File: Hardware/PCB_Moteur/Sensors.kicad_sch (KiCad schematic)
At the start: 18 parts, among them J18 Screw_Terminal_01x04, J3 Screw_Terminal_01x04, U8 INA125UA/2K5, U9 MAX6612MXK

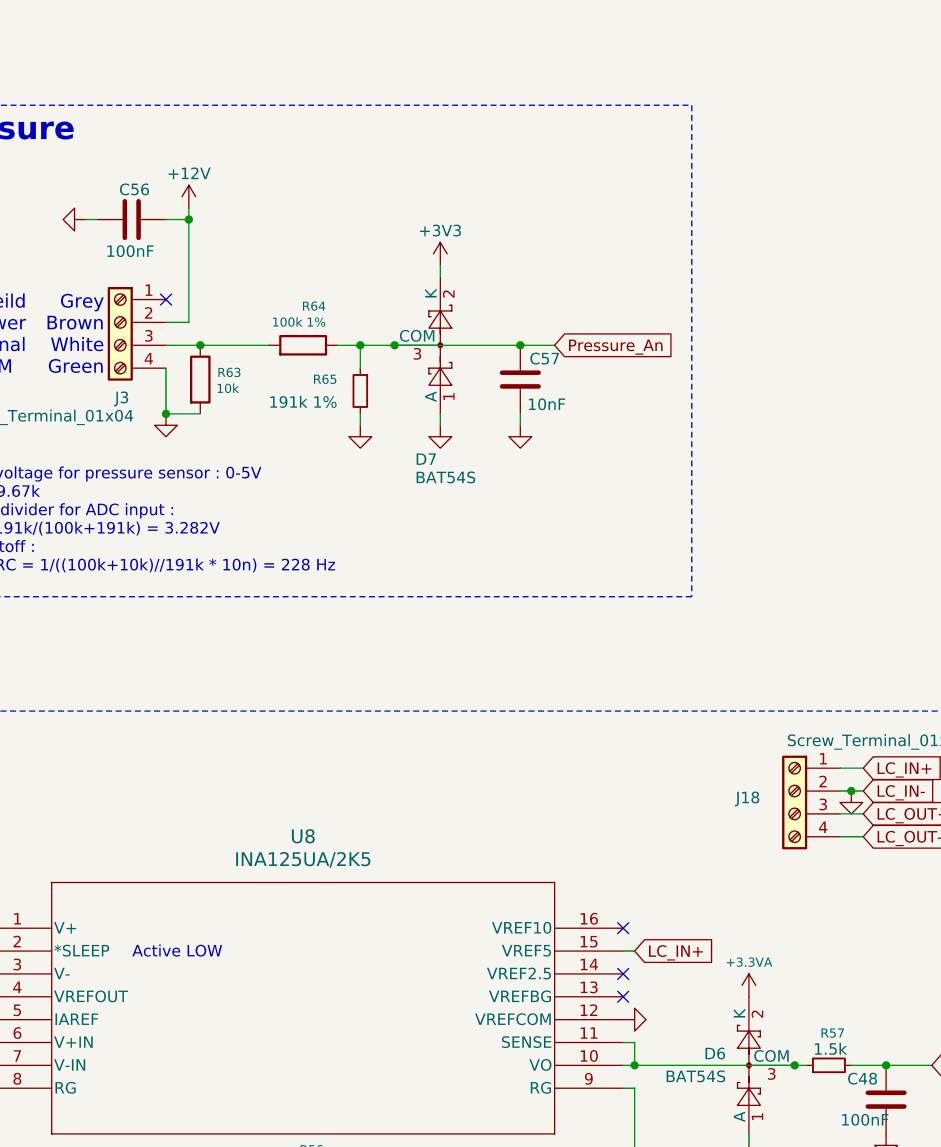
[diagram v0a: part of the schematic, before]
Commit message: wip: new pressure et fix alim
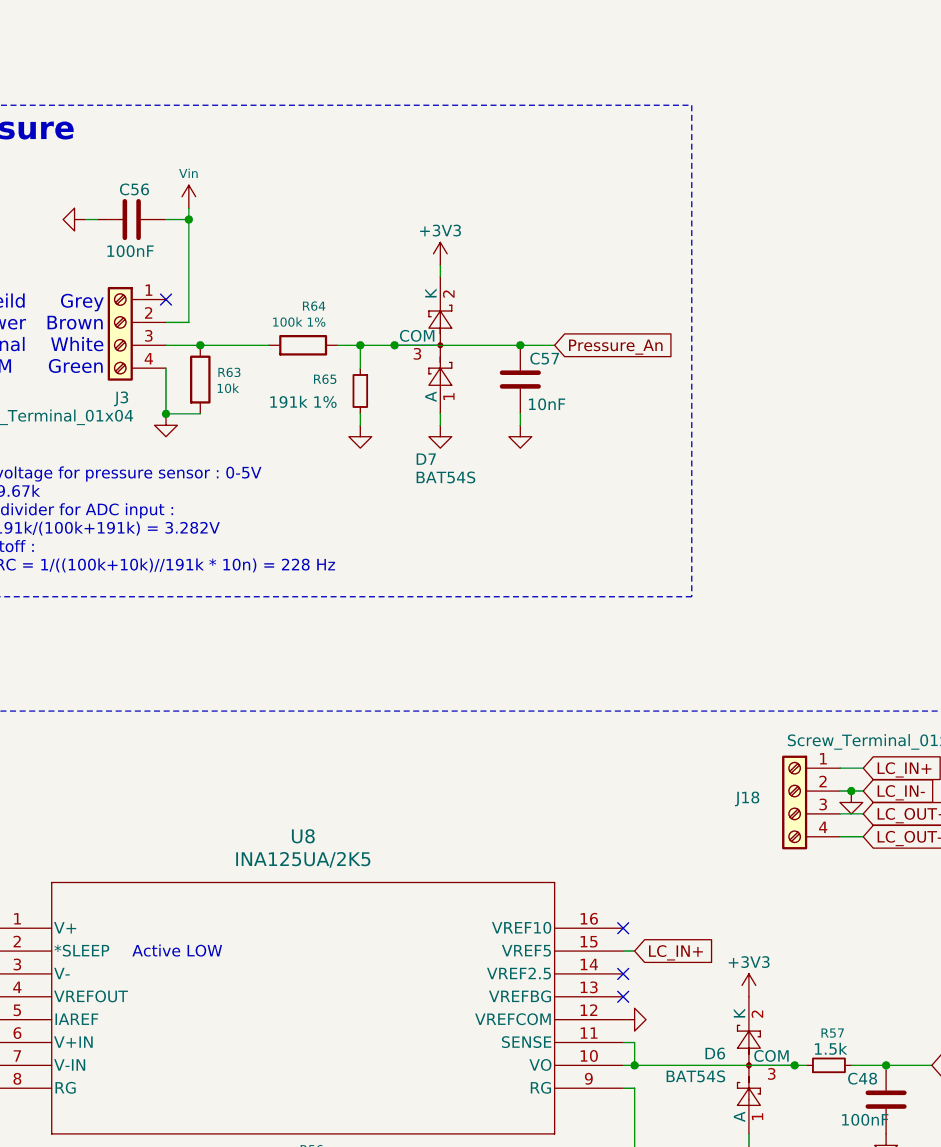
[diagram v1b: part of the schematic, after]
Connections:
- net +12V is gone; now on net Vin: C56.2, J3.2 (Pin_2)
- net +3.3VA is gone; now on net +3V3: D6.2 (K)
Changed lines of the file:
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@@
 	)
 	(symbol
-		(lib_id "power:+3.3VA")
+		(lib_id "power:+3V3")
 		(at 127 133.35 0)
-		(unit 1)
-		(exclude_from_sim no)
-		(in_bom yes)
-		(on_board yes)
-		(dnp no)
-		(property "Reference" "#PWR075"
+		(mirror y)
+		(unit 1)
+		(exclude_from_sim no)
+		(in_bom yes)
+		(on_board yes)
+		(dnp no)
+		(property "Reference" "#PWR037"
 			(at 127 137.16 0)
 			(effects
 				(font
-					(size 1 1)
-				)
-				(hide yes)
-			)
-		)
-		(property "Value" "+3.3VA"
+					(size 1.27 1.27)
+				)
+				(hide yes)
+			)
+		)
+		(property "Value" "+3V3"
 			(at 127 129.54 0)
 			(effects
 				(font
-					(size 1 1)
+					(size 1.27 1.27)
 				)
 			)
@@
 			(effects
 				(font
-					(size 1 1)
+					(size 1.27 1.27)
 				)
 				(hide yes)
@@
 			(effects
 				(font
-					(size 1 1)
-				)
-				(hide yes)
-			)
-		)
-		(property "Description" ""
+					(size 1.27 1.27)
+				)
+				(hide yes)
+			)
+		)
+		(property "Description" "Power symbol creates a global label with name \"+3V3\""
 			(at 127 133.35 0)
 			(effects
@@
 					(size 1.27 1.27)
 				)
-			)
-		)
-		(pin "1"
-		)
-		(instances
-			(project "PCB_moteur"
-				(path "/b0d87684-7b1c-41d8-8358-755aa327573e/f31687d3-ca84-4d71-914a-32b6c2b363a9"
-					(reference "#PWR075")
+				(hide yes)
+			)
+		)
+		(pin "1"
+		)
+		(instances
+			(project "PCB_moteur"
+				(path "/b0d87684-7b1c-41d8-8358-755aa327573e/f31687d3-ca84-4d71-914a-32b6c2b363a9"
+					(reference "#PWR037")
 					(unit 1)
 				)
@@
 	)
 	(symbol
-		(lib_name "+12V_1")
-		(lib_id "power:+12V")
-		(at 64.77 45.72 0)
-		(unit 1)
-		(exclude_from_sim no)
-		(in_bom yes)
-		(on_board yes)
-		(dnp no)
-		(property "Reference" "#PWR0146"
-			(at 64.77 49.53 0)
-			(effects
-				(font
-					(size 1.27 1.27)
-				)
-				(hide yes)
-			)
-		)
-		(property "Value" "+12V"
-			(at 64.77 41.91 0)
-			(effects
-				(font
-					(size 1.27 1.27)
-				)
-			)
-		)
-		(property "Footprint" ""
-			(at 64.77 45.72 0)
-			(effects
-				(font
-					(size 1.27 1.27)
-				)
-				(hide yes)
-			)
-		)
-		(property "Datasheet" ""
-			(at 64.77 45.72 0)
-			(effects
-				(font
-					(size 1.27 1.27)
-				)
-				(hide yes)
-			)
-		)
-		(property "Description" "Power symbol creates a global label with name \"+12V\""
-			(at 64.77 45.72 0)
-			(effects
-				(font
-					(size 1.27 1.27)
-				)
-				(hide yes)
-			)
-		)
-		(pin "1"
-		)
-		(instances
-			(project "PCB_moteur"
-				(path "/b0d87684-7b1c-41d8-8358-755aa327573e/f31687d3-ca84-4d71-914a-32b6c2b363a9"
-					(reference "#PWR0146")
-					(unit 1)
-				)
-			)
-		)
-	)
-	(symbol
 		(lib_id "power:GND")
 		(at 101.6 69.85 0)
@@
 					(unit 1)
 				)
+			)
+		)
+	)
+	(symbol
+		(lib_id "power:+12V")
+		(at 64.77 45.72 0)
+		(unit 1)
+		(exclude_from_sim no)
+		(in_bom yes)
+		(on_board yes)
+		(dnp no)
+		(property "Reference" "#PWR07"
+			(at 64.77 49.53 0)
+			(effects
+				(font
+					(size 1 1)
+				)
+				(hide yes)
+			)
+		)
+		(property "Value" "Vin"
+			(at 64.77 41.91 0)
+			(effects
+				(font
+					(size 1 1)
+				)
+			)
+		)
+		(property "Footprint" ""
+			(at 64.77 45.72 0)
+			(effects
+				(font
+					(size 1 1)
+				)
+				(hide yes)
+			)
+		)
+		(property "Datasheet" ""
+			(at 64.77 45.72 0)
+			(effects
+				(font
+					(size 1 1)
+				)
+				(hide yes)
+			)
+		)
+		(property "Description" ""
+			(at 64.77 45.72 0)
+			(effects
+				(font
+					(size 1.27 1.27)
+				)
+				(hide yes)
+			)
+		)
+		(pin "1"
+		)
+		(instances
+			(project "PCB_moteur"
+				(path "/b0d87684-7b1c-41d8-8358-755aa327573e/f31687d3-ca84-4d71-914a-32b6c2b363a9"
+					(reference "#PWR07")
+					(unit 1)
+				)
